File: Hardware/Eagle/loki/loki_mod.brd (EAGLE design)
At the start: 21.9 x 22.9 mm, 39 parts

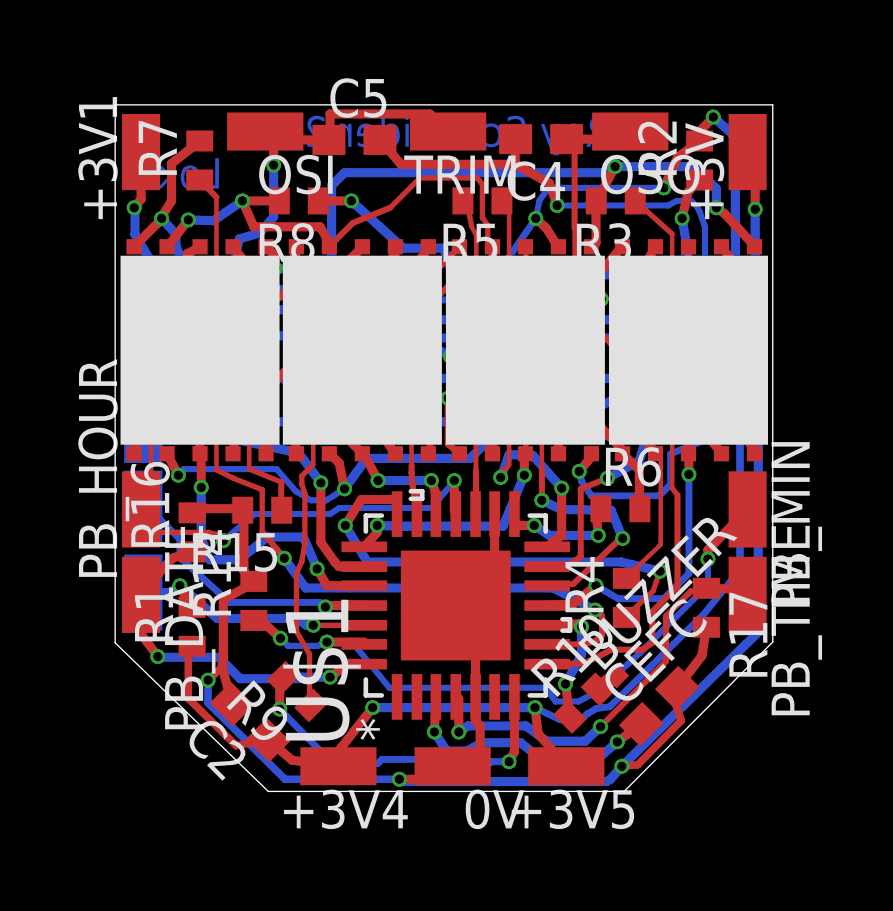
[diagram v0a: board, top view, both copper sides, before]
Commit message: Reviewed boards and code.
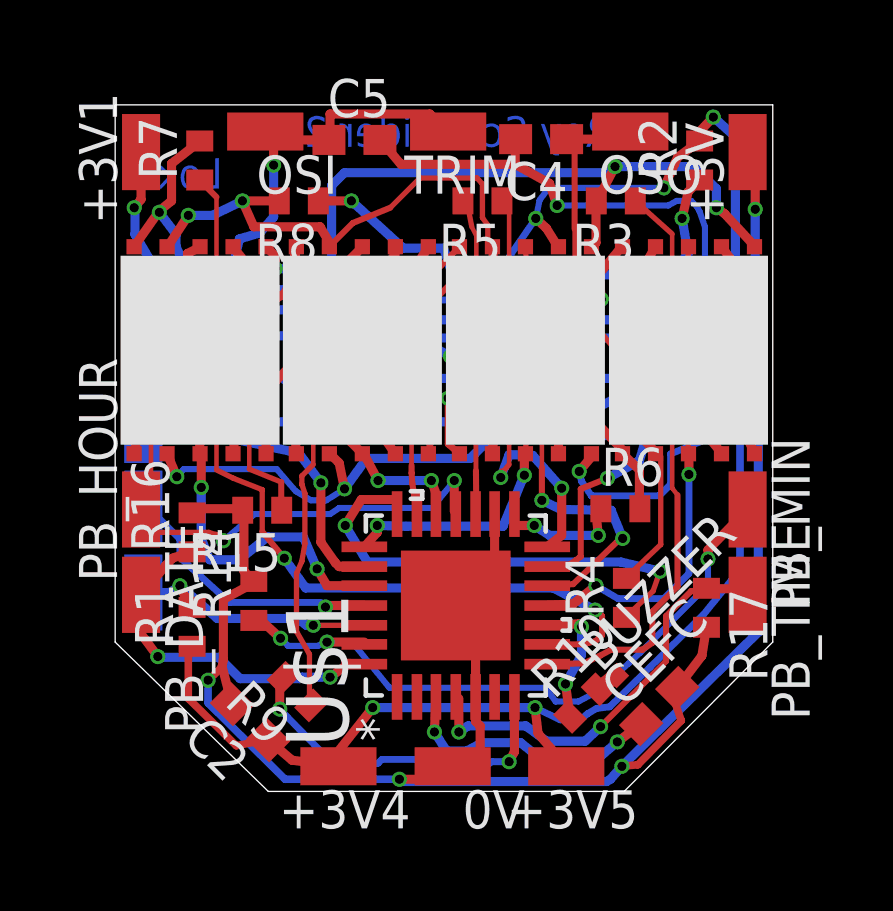
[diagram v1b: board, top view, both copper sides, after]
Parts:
- R10: value 680 -> 470
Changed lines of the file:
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@@
 <plain>
 <wire x1="5.08" y1="-0.1524" x2="16.9418" y2="-0.1524" width="0" layer="20"/>
-<wire x1="-0.0254" y1="4.8006" x2="5.08" y2="-0.1524" width="0" layer="20"/>
+<wire x1="-0.0254" y1="4.826" x2="5.08" y2="-0.1524" width="0" layer="20"/>
 <wire x1="16.9418" y1="-0.1524" x2="21.8948" y2="4.826" width="0" layer="20"/>
 <wire x1="21.8948" y1="4.826" x2="21.8948" y2="22.733" width="0" layer="20"/>
 <wire x1="21.8948" y1="22.733" x2="0" y2="22.733" width="0" layer="20"/>
-<wire x1="-0.0254" y1="22.723" x2="-0.0254" y2="4.8006" width="0" layer="20"/>
+<wire x1="-0.0254" y1="22.733" x2="-0.0254" y2="4.826" width="0" layer="20"/>
 <text x="16.51" y="21.336" size="1.016" layer="16" font="vector" ratio="16" rot="MR0">Roy Schneider 2021</text>
 <text x="3.556" y="19.939" size="1.016" layer="16" font="vector" ratio="16" rot="MR0">Loki</text>
@@
 <element name="1M" library="l104g" package="L104G" value="L104G" x="16.5862" y="11.4046"/>
 <element name="R9" library="resistor" package="R0402" value="100/130" x="6.0452" y="3.175" rot="R135"/>
-<element name="R10" library="resistor" package="R0402" value="680" x="15.5956" y="2.794" rot="R45"/>
+<element name="R10" library="resistor" package="R0402" value="470" x="15.5956" y="2.794" rot="R45"/>
 <element name="BUZZER" library="testpad" package="TP06SQ" value="TPTP06SQ" x="16.6878" y="3.7084" rot="R45">
 <attribute name="TP_SIGNAL_NAME" value="" x="16.6878" y="3.7084" size="1.778" layer="27" rot="R45" display="off"/>
@@
 <wire x1="9.3726" y1="9.5758" x2="8.1788" y2="9.5758" width="0.3048" layer="1"/>
 <wire x1="9.3726" y1="9.0932" x2="9.3726" y2="9.5758" width="0.3048" layer="1"/>
-<wire x1="16.9926" y1="5.6642" x2="17.018" y2="5.6492" width="0.1524" layer="1"/>
+<wire x1="16.9926" y1="5.6642" x2="17.018" y2="5.6492" width="0.1778" layer="1"/>
 <via x="18.1356" y="7.1882" extent="1-16" drill="0.3048"/>
 <via x="7.6454" y="8.7122" extent="1-16" drill="0.3048"/>
@@
 <wire x1="17.8816" y1="4.8006" x2="17.5514" y2="4.572" width="0.2032" layer="1"/>
 <wire x1="14.3764" y1="4.0894" x2="15.5956" y2="4.1148" width="0.2032" layer="1"/>
-<wire x1="18.542" y1="9.9568" x2="18.7198" y2="9.7282" width="0.1778" layer="1"/>
+<wire x1="18.542" y1="9.9568" x2="18.7198" y2="9.7282" width="0.1524" layer="1"/>
 <wire x1="18.7198" y1="9.7282" x2="18.7198" y2="6.6802" width="0.2032" layer="1"/>
 <wire x1="18.542" y1="9.9568" x2="18.542" y2="12.4968" width="0.1524" layer="1"/>
@@
 <contactref element="R17" pad="1"/>
 <wire x1="21.1074" y1="6.604" x2="19.685" y2="6.604" width="0.3048" layer="1"/>
-<wire x1="21.0566" y1="6.4008" x2="21.1074" y2="6.604" width="0.1524" layer="1"/>
+<wire x1="21.0566" y1="6.4008" x2="21.1074" y2="6.604" width="0.3048" layer="1"/>
 <wire x1="19.685" y1="6.604" x2="19.685" y2="6.619" width="0.1524" layer="1"/>
 <wire x1="11.43" y1="2.9464" x2="11.3284" y2="2.9972" width="0.1524" layer="1"/>
@@
 <contactref element="1M" pad="10F"/>
 <contactref element="R7" pad="2"/>
-<wire x1="1.8542" y1="19.5326" x2="1.397" y2="18.796" width="0.3048" layer="1"/>
-<wire x1="1.397" y1="18.796" x2="0.6096" y2="18.0086" width="0.3048" layer="1"/>
+<wire x1="1.8542" y1="19.5326" x2="1.4478" y2="19.2024" width="0.3048" layer="1"/>
+<wire x1="1.4478" y1="19.2024" x2="0.6096" y2="18.0086" width="0.3048" layer="1"/>
 <wire x1="1.8542" y1="20.7772" x2="1.8542" y2="19.5326" width="0.3048" layer="1"/>
 <wire x1="2.794" y1="21.5138" x2="1.8542" y2="20.7772" width="0.3048" layer="1"/>
@@
 <wire x1="4.8514" y1="16.0274" x2="5.6134" y2="16.4338" width="0.3048" layer="1"/>
 <wire x1="5.9944" y1="17.9832" x2="6.015" y2="18.0046" width="0.1524" layer="1"/>
-<wire x1="1.524" y1="18.9484" x2="1.397" y2="18.796" width="0.3048" layer="1"/>
+<wire x1="1.4478" y1="19.1516" x2="1.4478" y2="19.2024" width="0.3048" layer="1"/>
 <wire x1="9.4996" y1="15.9766" x2="11.43" y2="17.9832" width="0.2032" layer="1"/>
 <wire x1="11.43" y1="17.9832" x2="11.4506" y2="18.0046" width="0.1524" layer="1"/>
@@
 <wire x1="16.8656" y1="18.0086" x2="16.8862" y2="18.0046" width="0.1524" layer="1"/>
 <via x="4.8514" y="16.0274" extent="1-16" drill="0.3048"/>
-<via x="1.524" y="18.9484" extent="1-16" drill="0.3048"/>
+<via x="1.4478" y="19.1516" extent="1-16" drill="0.3048"/>
 <via x="9.4996" y="15.9766" extent="1-16" drill="0.3048"/>
 <via x="16.1798" y="16.256" extent="1-16" drill="0.3048"/>
 <wire x1="2.794" y1="16.1798" x2="2.0066" y2="18.0086" width="0.3048" layer="16"/>
 <wire x1="2.0066" y1="18.0086" x2="2.0066" y2="18.415" width="0.3048" layer="16"/>
-<wire x1="2.0066" y1="18.415" x2="1.524" y2="18.9484" width="0.3048" layer="16"/>
+<wire x1="2.0066" y1="18.415" x2="1.4478" y2="19.1516" width="0.3048" layer="16"/>
 <wire x1="5.3594" y1="15.9004" x2="4.8514" y2="16.0274" width="0.3048" layer="16"/>
 <wire x1="9.4996" y1="15.9766" x2="8.6106" y2="15.9004" width="0.3048" layer="16"/>
@@
 <contactref element="1M" pad="9G"/>
 <contactref element="R8" pad="2"/>
-<wire x1="2.413" y1="18.8976" x2="1.7272" y2="18.0086" width="0.3048" layer="1"/>
+<wire x1="2.413" y1="19.05" x2="1.7272" y2="18.0086" width="0.3048" layer="1"/>
 <wire x1="5.4356" y1="19.5326" x2="4.2164" y2="19.5326" width="0.3048" layer="1"/>
 <wire x1="1.7272" y1="18.0086" x2="1.7048" y2="18.0046" width="0.1524" layer="1"/>
@@
 <wire x1="17.9832" y1="18.0086" x2="17.9862" y2="18.0046" width="0.1524" layer="1"/>
 <wire x1="12.573" y1="17.9324" x2="12.5506" y2="18.0046" width="0.1524" layer="1"/>
-<via x="2.413" y="18.8976" extent="1-16" drill="0.3048"/>
+<via x="2.413" y="19.05" extent="1-16" drill="0.3048"/>
 <via x="4.2164" y="19.5326" extent="1-16" drill="0.3048"/>
 <via x="17.4498" y="17.0688" extent="1-16" drill="0.3048"/>
 <via x="12.573" y="16.764" extent="1-16" drill="0.3048"/>
-<wire x1="4.2164" y1="19.5326" x2="3.2512" y2="18.8722" width="0.3048" layer="16"/>
-<wire x1="3.2512" y1="18.8722" x2="2.413" y2="18.8976" width="0.3048" layer="16"/>
+<wire x1="4.2164" y1="19.5326" x2="3.2258" y2="19.05" width="0.3048" layer="16"/>
+<wire x1="3.2258" y1="19.05" x2="2.413" y2="19.05" width="0.3048" layer="16"/>
 <wire x1="7.1628" y1="18.0594" x2="6.8072" y2="18.669" width="0.3048" layer="1"/>
 <wire x1="6.8072" y1="18.669" x2="4.5974" y2="18.669" width="0.3048" layer="1"/>
@@
 <contactref element="R4" pad="2"/>
 <wire x1="18.161" y1="11.0236" x2="18.0086" y2="11.1252" width="0.1524" layer="1"/>
-<wire x1="18.161" y1="8.0772" x2="18.161" y2="11.0236" width="0.1524" layer="1"/>
-<wire x1="16.9926" y1="6.9596" x2="18.161" y2="8.0772" width="0.1524" layer="1"/>
+<wire x1="18.161" y1="8.0772" x2="18.161" y2="11.0236" width="0.1778" layer="1"/>
+<wire x1="16.9926" y1="6.9596" x2="18.161" y2="8.0772" width="0.1778" layer="1"/>
 <wire x1="18.0086" y1="11.1252" x2="17.9862" y2="11.1046" width="0.1524" layer="1"/>
-<wire x1="16.9926" y1="6.9596" x2="17.018" y2="6.9492" width="0.1524" layer="1"/>
+<wire x1="16.9926" y1="6.9596" x2="17.018" y2="6.9492" width="0.1778" layer="1"/>
 <wire x1="6.5024" y1="9.5504" x2="5.9944" y2="9.8552" width="0.2032" layer="16"/>
 <wire x1="7.0104" y1="9.5504" x2="6.5024" y2="9.5504" width="0.2032" layer="16"/>
@@
 <wire x1="17.9578" y1="11.2014" x2="17.9862" y2="11.1046" width="0.1524" layer="1"/>
 <wire x1="12.7254" y1="11.7856" x2="12.6746" y2="11.811" width="0.1524" layer="16"/>
-<via x="2.0828" y="10.3886" extent="1-16" drill="0.3048"/>
+<via x="2.032" y="10.3378" extent="1-16" drill="0.3048"/>
 <via x="7.62" y="9.9314" extent="1-16" drill="0.3048"/>
 <via x="12.6746" y="11.811" extent="1-16" drill="0.3048"/>
 <via x="17.0688" y="12.2174" extent="1-16" drill="0.3048"/>
-<wire x1="2.0828" y1="10.3886" x2="2.2606" y2="10.5918" width="0.2032" layer="16"/>
+<wire x1="2.032" y1="10.3378" x2="2.2606" y2="10.5918" width="0.2032" layer="16"/>
 <wire x1="2.2606" y1="10.5918" x2="5.3594" y2="10.5918" width="0.2032" layer="16"/>
 <wire x1="5.9944" y1="9.8552" x2="5.3594" y2="10.5918" width="0.2032" layer="16"/>
@@
 <wire x1="16.4846" y1="11.7094" x2="12.827" y2="11.7094" width="0.3048" layer="16"/>
 <wire x1="12.827" y1="11.7094" x2="12.6746" y2="11.811" width="0.3048" layer="16"/>
-<wire x1="1.7048" y1="11.1046" x2="2.0828" y2="10.3886" width="0.3048" layer="1"/>
+<wire x1="1.7048" y1="11.1046" x2="2.032" y2="10.3378" width="0.3048" layer="1"/>
 </signal>
 <signal name="N$8">
